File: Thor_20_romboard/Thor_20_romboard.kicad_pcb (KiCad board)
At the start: 2 copper layers, 47 x 128.3 mm, 13 parts, among them J1 EPROM CARD, U1 27128, U2 27128, U3 27256, U4 27256, U5 27256, U6 2764

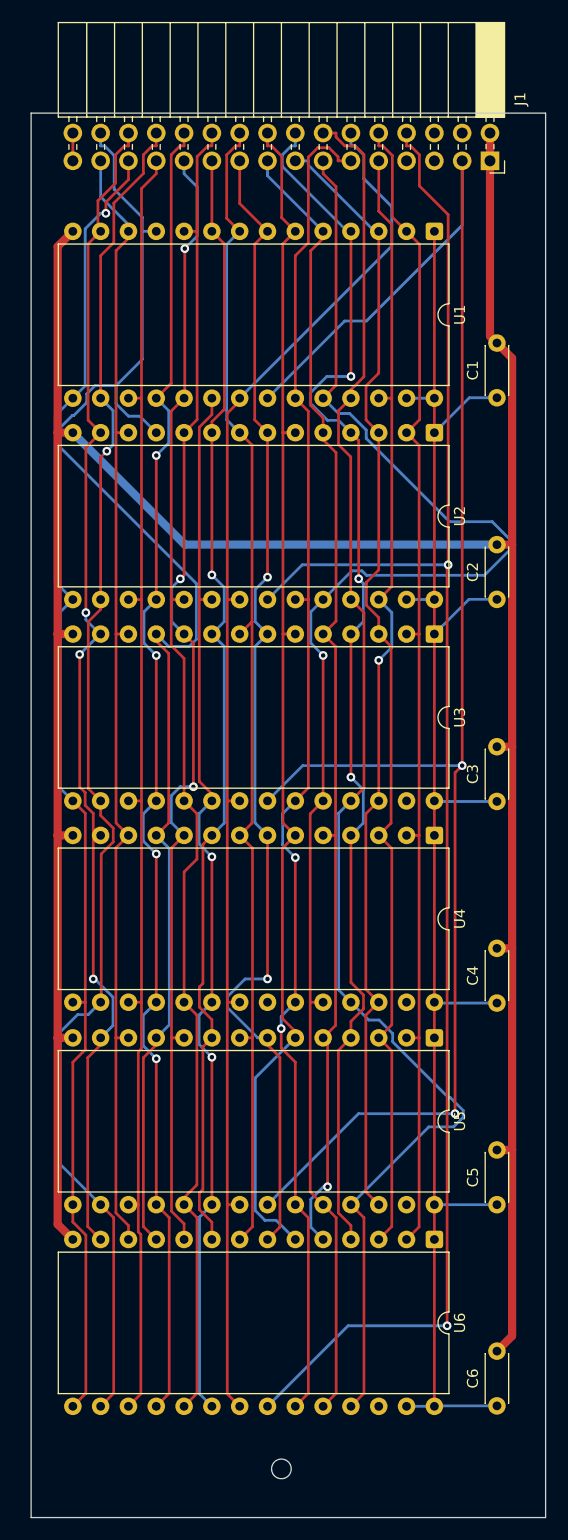
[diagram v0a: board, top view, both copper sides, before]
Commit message: add 3D and good romboard
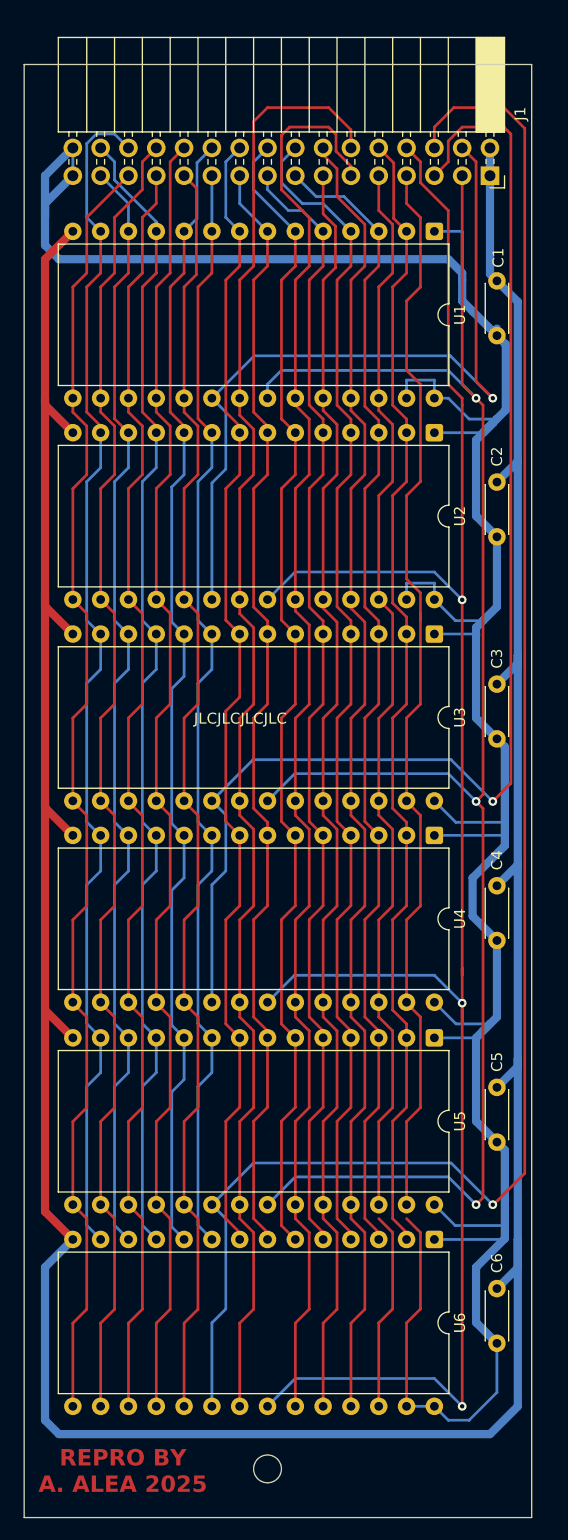
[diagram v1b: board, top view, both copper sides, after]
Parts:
- moved C3 5.72 mm to (192.4, 139.7)
- moved C4 5.72 mm to (192.4, 158.1)
- moved C5 5.72 mm to (192.4, 176.5)
- moved C6 5.72 mm to (192.4, 194.9)
- moved C2 5.71 mm to (192.4, 121.2)
- moved C1 5.67 mm to (192.4, 102.9)
- moved J1 1.36 mm to (191.8, 88.3)
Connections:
- U3 pad 20: /NS1 -> /NS2
- U3 pad 27: unconnected-(U3-A14-Pad27) -> /A14
- U4 pad 20: /NS1 -> /NS2
- U4 pad 22: unconnected-(U4-~{OE}-Pad22) -> /A15'
- U4 pad 27: unconnected-(U4-A14-Pad27) -> /A14
- U5 pad 20: /NS1 -> /NS3
- U5 pad 27: unconnected-(U5-A14-Pad27) -> /A14
- U6 pad 20: /NS1 -> /NS3
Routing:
- net /NS3: track 0.00 -> 159.5 mm, vias 0 -> 1
- net +5V: track 154.5 -> 276.9 mm
- net /NS2: track 0.00 -> 120.1 mm, vias 0 -> 1
- net /A14: track 0.00 -> 99.8 mm
- net GND: track 259.9 -> 306.8 mm
- net /A15': track 148.0 -> 178.6 mm, vias 2 -> 3
- net /A9: track 143.5 -> 118.6 mm, vias 1 -> 0
- net /NS1: track 97.0 -> 72.3 mm, vias 2 -> 1
- net /D0: track 127.8 -> 106.9 mm
- net unconnected-(U6-NC-Pad26): track 0.00 -> 18.2 mm
- net /A8: track 133.9 -> 122.4 mm
- net /A11: track 124.7 -> 132.9 mm, vias 2 -> 0
- net /A10: track 129.3 -> 135.1 mm
- net /A3: track 108.1 -> 103.5 mm, vias 2 -> 0
- net /A6: track 113.3 -> 109.2 mm, vias 3 -> 0
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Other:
- board size 47 x 128.3 mm -> 46.4 x 132.7 mm
- board text added: "JLCJLCJLCJLC"
- board text added: "REPRO BY A. ALEA 2025"
